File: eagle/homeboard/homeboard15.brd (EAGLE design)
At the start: 100 x 80 mm, 122 parts, among them IC1 XCF02S, IC2 25LC080SN, IC3 ATMEGA32U2-TQFP, Q5 BC848SMD, Q6 BC848SMD, Q7 BC848SMD, Q8 BC848SMD, T1 BSS138, T2 BC848, T3 BSS138, U1 XC3S400TQ144, X1 1503_04, X2 SCART-F, X6 MINI-USB_4P-85-32004-10X, X7 DC21MMX

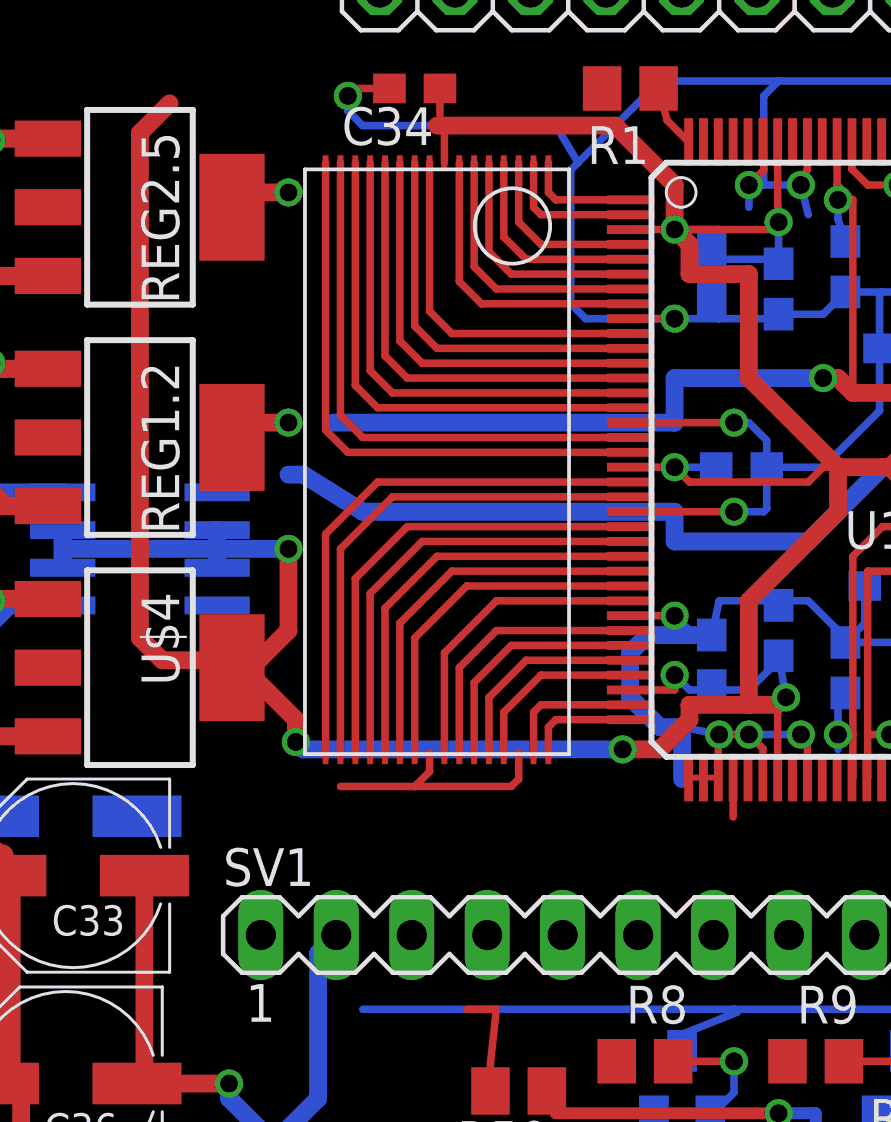
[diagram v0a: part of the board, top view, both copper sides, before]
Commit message: mah
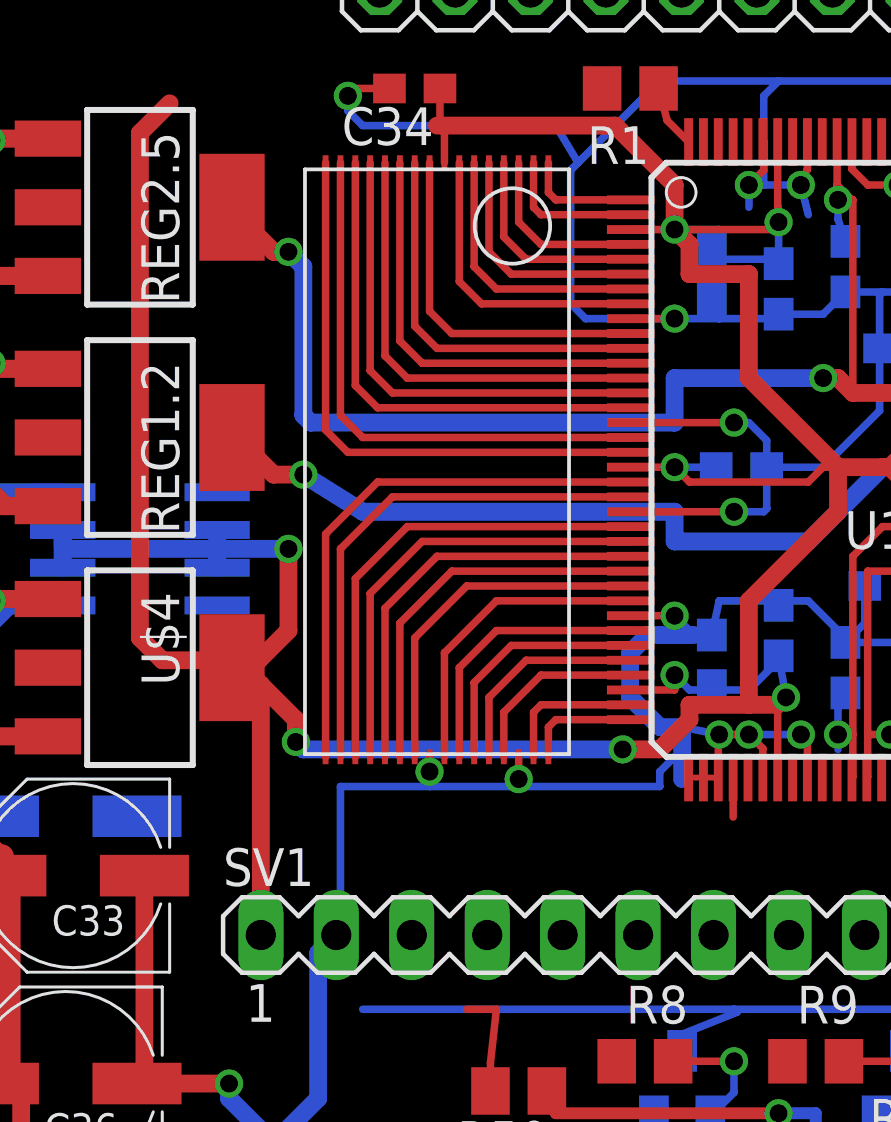
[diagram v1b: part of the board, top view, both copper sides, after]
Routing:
- net GND: track 653.0 -> 664.9 mm, vias 33 -> 35
- net VCC: track 389.0 -> 398.4 mm
- net VCCAUX: track 89.2 -> 95.8 mm
- net VCCINT: track 82.1 -> 81.1 mm
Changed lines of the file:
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@@
 <contactref element="U$6" pad="P30"/>
 <wire x1="21.25" y1="31" x2="21.25" y2="30.25" width="0.254" layer="1"/>
-<wire x1="18.25" y1="30.5" x2="17.75" y2="30" width="0.254" layer="1"/>
-<wire x1="17.75" y1="30" x2="15.25" y2="30" width="0.254" layer="1"/>
-<wire x1="21.25" y1="30.25" x2="21" y2="30" width="0.254" layer="1"/>
-<wire x1="21" y1="30" x2="17.75" y2="30" width="0.254" layer="1"/>
 <contactref element="C34" pad="2"/>
 <wire x1="16.9" y1="53.5" x2="15.75" y2="53.5" width="0.254" layer="1"/>
@@
 <wire x1="25" y1="33" x2="26" y2="32" width="0.6" layer="16"/>
 <wire x1="26" y1="32" x2="26.75" y2="32" width="0.6" layer="16"/>
+<via x="21.25" y="30.25" extent="1-16" drill="0.6" shape="square"/>
+<wire x1="21.25" y1="30.25" x2="21.25" y2="30" width="0.254" layer="16"/>
+<wire x1="21.25" y1="30" x2="18.25" y2="30" width="0.254" layer="16"/>
+<via x="18.25" y="30.5" extent="1-16" drill="0.6" shape="square"/>
+<wire x1="18.25" y1="30.5" x2="18.25" y2="30" width="0.254" layer="16"/>
+<wire x1="18.25" y1="30" x2="15.25" y2="30" width="0.254" layer="16"/>
+<wire x1="15.25" y1="30" x2="15.25" y2="25.14" width="0.254" layer="16"/>
+<wire x1="15.25" y1="25.14" x2="15.11" y2="25" width="0.254" layer="16"/>
+<wire x1="26" y1="30" x2="21.5" y2="30" width="0.254" layer="16"/>
+<wire x1="21.5" y1="30" x2="21.25" y2="30.25" width="0.254" layer="16"/>
+<wire x1="26" y1="30" x2="26" y2="30.5" width="0.254" layer="16"/>
+<wire x1="26" y1="30.5" x2="26.5" y2="31" width="0.254" layer="16"/>
+<wire x1="26.75" y1="30.25" x2="26.75" y2="30.75" width="0.254" layer="16"/>
+<wire x1="26.75" y1="30.75" x2="26.5" y2="31" width="0.254" layer="16"/>
 <wire x1="80.3716" y1="70.77" x2="97" y2="76.3" width="0" layer="19" extent="1-1"/>
 <wire x1="71.4890875" y1="62.801446875" x2="80.3716" y2="70.77" width="0" layer="19" extent="1-1"/>
@@
 <wire x1="41.97" y1="51.7" x2="42" y2="51.75" width="0" layer="19" extent="1-1"/>
 <wire x1="29.47" y1="51.7" x2="29.5" y2="51.75" width="0" layer="19" extent="1-1"/>
-<wire x1="21.25" y1="31" x2="25" y2="33" width="0" layer="19" extent="1-16"/>
-<wire x1="15.11" y1="25" x2="15.25" y2="30" width="0" layer="19" extent="1-1"/>
 <wire x1="56.335" y1="7.5" x2="56.5" y2="7.5" width="0" layer="19" extent="1-1"/>
 <wire x1="8.4" y1="29" x2="8.65" y2="27" width="0" layer="19" extent="1-16"/>
@@
 <via x="13.75" y="31.5" extent="1-16" drill="0.6" shape="square"/>
 <wire x1="13.75" y1="31.5" x2="13.75" y2="32.25" width="0.6" layer="1"/>
-<wire x1="13.75" y1="32.25" x2="12" y2="34" width="0.6" layer="1"/>
+<wire x1="13.75" y1="32.25" x2="12.57" y2="33.43" width="0.6" layer="1"/>
+<wire x1="12.57" y1="25" x2="12.57" y2="33.43" width="0.6" layer="1"/>
+<wire x1="12.57" y1="33.43" x2="12" y2="34" width="0.6" layer="1"/>
+<wire x1="12" y1="34" x2="11.5" y2="34" width="0.6" layer="1"/>
+<wire x1="11.5" y1="34" x2="11.5" y2="33.5" width="0.6" layer="1"/>
 <wire x1="88.7" y1="64.0426" x2="89.5" y2="64.0426" width="0" layer="19" extent="1-1"/>
 <wire x1="87.2074" y1="60.15" x2="88.7" y2="64.0426" width="0" layer="19" extent="1-1"/>
 <wire x1="75.5" y1="52.25" x2="87.2074" y2="60.15" width="0" layer="19" extent="1-1"/>
-<wire x1="11.599" y1="34" x2="12" y2="34" width="0" layer="19" extent="1-1"/>
-<wire x1="12.57" y1="25" x2="14" y2="31.25" width="0" layer="19" extent="16-16"/>
+<wire x1="11.599" y1="34" x2="11.5" y2="34" width="0" layer="19" extent="1-1"/>
 <wire x1="16" y1="22.5" x2="12.57" y2="25" width="0" layer="19" extent="16-16"/>
 <wire x1="66.2890875" y1="58.991446875" x2="67" y2="52.25" width="0" layer="19" extent="1-1"/>
@@
 <wire x1="37" y1="44.25" x2="38" y2="45.25" width="0.6" layer="1"/>
 <wire x1="38" y1="45.25" x2="38" y2="50.25" width="0.6" layer="1"/>
-<via x="13.5" y="42.25" extent="1-16" drill="0.6" shape="square"/>
 <wire x1="26.5" y1="39.25" x2="26.5" y2="38.25" width="0.6" layer="16"/>
 <wire x1="26.5" y1="38.25" x2="31" y2="38.25" width="0.6" layer="16"/>
 <wire x1="31" y1="38.25" x2="33.5" y2="40.75" width="0.6" layer="16"/>
 <wire x1="33.5" y1="40.75" x2="37" y2="40.75" width="0.6" layer="16"/>
-<wire x1="11" y1="42.349" x2="11.599" y2="41.75" width="0.6" layer="1"/>
 <wire x1="26.5" y1="39.25" x2="16" y2="39.25" width="0.6" layer="16"/>
 <wire x1="16" y1="39.25" x2="14" y2="40.5" width="0.6" layer="16"/>
-<wire x1="14" y1="40.5" x2="13.5" y2="40.5" width="0.6" layer="16"/>
-<wire x1="13.5" y1="40.5" x2="14.75" y2="39.25" width="0" layer="19" extent="1-16"/>
-<wire x1="14.5" y1="39.25" x2="15.25" y2="39.25" width="0" layer="19" extent="1-16"/>
-<wire x1="14.75" y1="39.25" x2="14.5" y2="39.25" width="0" layer="19" extent="1-16"/>
-<wire x1="13.5" y1="42.25" x2="11.25" y2="42.25" width="0.6" layer="1"/>
-<wire x1="11.25" y1="42.25" x2="11" y2="42.5" width="0.6" layer="1"/>
-<wire x1="11" y1="42.349" x2="11" y2="42.5" width="0.6" layer="1"/>
+<via x="14" y="40.5" extent="1-16" drill="0.6" shape="square"/>
+<wire x1="14" y1="40.5" x2="13" y2="40.5" width="0.6" layer="1"/>
+<wire x1="13" y1="40.5" x2="11.5" y2="42" width="0.6" layer="1"/>
 <wire x1="38.5" y1="51.75" x2="38.47" y2="51.7" width="0" layer="19" extent="1-1"/>
-<wire x1="13.5" y1="42.25" x2="14.5" y2="39.25" width="0" layer="19" extent="16-16"/>
+<wire x1="11.599" y1="41.75" x2="11.5" y2="42" width="0" layer="19" extent="1-1"/>
 </signal>
 <signal name="VCCAUX">
@@
 <wire x1="32.5" y1="37.75" x2="33.5" y2="38.75" width="0.254" layer="1"/>
 <wire x1="33.5" y1="38.75" x2="39.5" y2="38.75" width="0.254" layer="1"/>
-<via x="13.5" y="50" extent="1-16" drill="0.6" shape="square"/>
 <wire x1="26.5" y1="42.25" x2="26.5" y2="43.75" width="0.6" layer="16"/>
 <wire x1="26.5" y1="43.75" x2="31.5" y2="43.75" width="0.6" layer="16"/>
@@
 <wire x1="39" y1="47.85" x2="39" y2="49.25" width="0.254" layer="16"/>
 <wire x1="11" y1="48.75" x2="11.5" y2="49.25" width="0.6" layer="1"/>
-<wire x1="26.5" y1="42.25" x2="15" y2="42.25" width="0.6" layer="16"/>
+<wire x1="26.5" y1="42.25" x2="14.25" y2="42.25" width="0.6" layer="16"/>
 <wire x1="11.5" y1="49.25" x2="12" y2="49.25" width="0.6" layer="1"/>
 <wire x1="12" y1="49.25" x2="12" y2="49" width="0.6" layer="1"/>
 <wire x1="12" y1="49" x2="11.599" y2="49" width="0.6" layer="1"/>
 <wire x1="11.599" y1="49" x2="11.599" y2="49.5" width="0.6" layer="1"/>
-<wire x1="13.5" y1="50" x2="12.099" y2="50" width="0.6" layer="1"/>
-<wire x1="12.099" y1="50" x2="11.599" y2="49.5" width="0.6" layer="1"/>
 <wire x1="32" y1="31.25" x2="32" y2="31.75" width="0.254" layer="16"/>
 <wire x1="20.3" y1="19.75" x2="20.3" y2="20.7" width="0.254" layer="1"/>
 <wire x1="20.3" y1="20.7" x2="20.5" y2="22.5" width="0.254" layer="1"/>
 <wire x1="20.5" y1="22.5" x2="19.5" y2="22.5" width="0.254" layer="1"/>
-<wire x1="15" y1="42.25" x2="12" y2="49" width="0" layer="19" extent="1-16"/>
+<wire x1="14.25" y1="42.25" x2="14" y2="42.5" width="0.6" layer="16"/>
+<wire x1="14" y1="42.5" x2="14" y2="47.5" width="0.6" layer="16"/>
+<wire x1="14" y1="47.5" x2="13.5" y2="48" width="0.6" layer="16"/>
+<via x="13.5" y="48" extent="1-16" drill="0.6" shape="square"/>
+<wire x1="13.5" y1="48" x2="13" y2="48" width="0.6" layer="1"/>
+<wire x1="13" y1="48" x2="12" y2="49" width="0.6" layer="1"/>
 <wire x1="20.5" y1="22.5" x2="32.47" y2="30.3" width="0" layer="19" extent="1-1"/>
 </signal>
